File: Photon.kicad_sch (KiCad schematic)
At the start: 58 parts, among them J1 USB_C_Receptacle_USB2.0_14P, Q1 IRLML6402, Q2 IRLML6402, SW1 TS-1088-AR02016, U1 ATtiny13A-S, U2 RT8059GJ5, U3 TP4056, U4 BCR421UW6-7, U5 DW01A, U6 FS8205A, U7 BCR421UW6-7

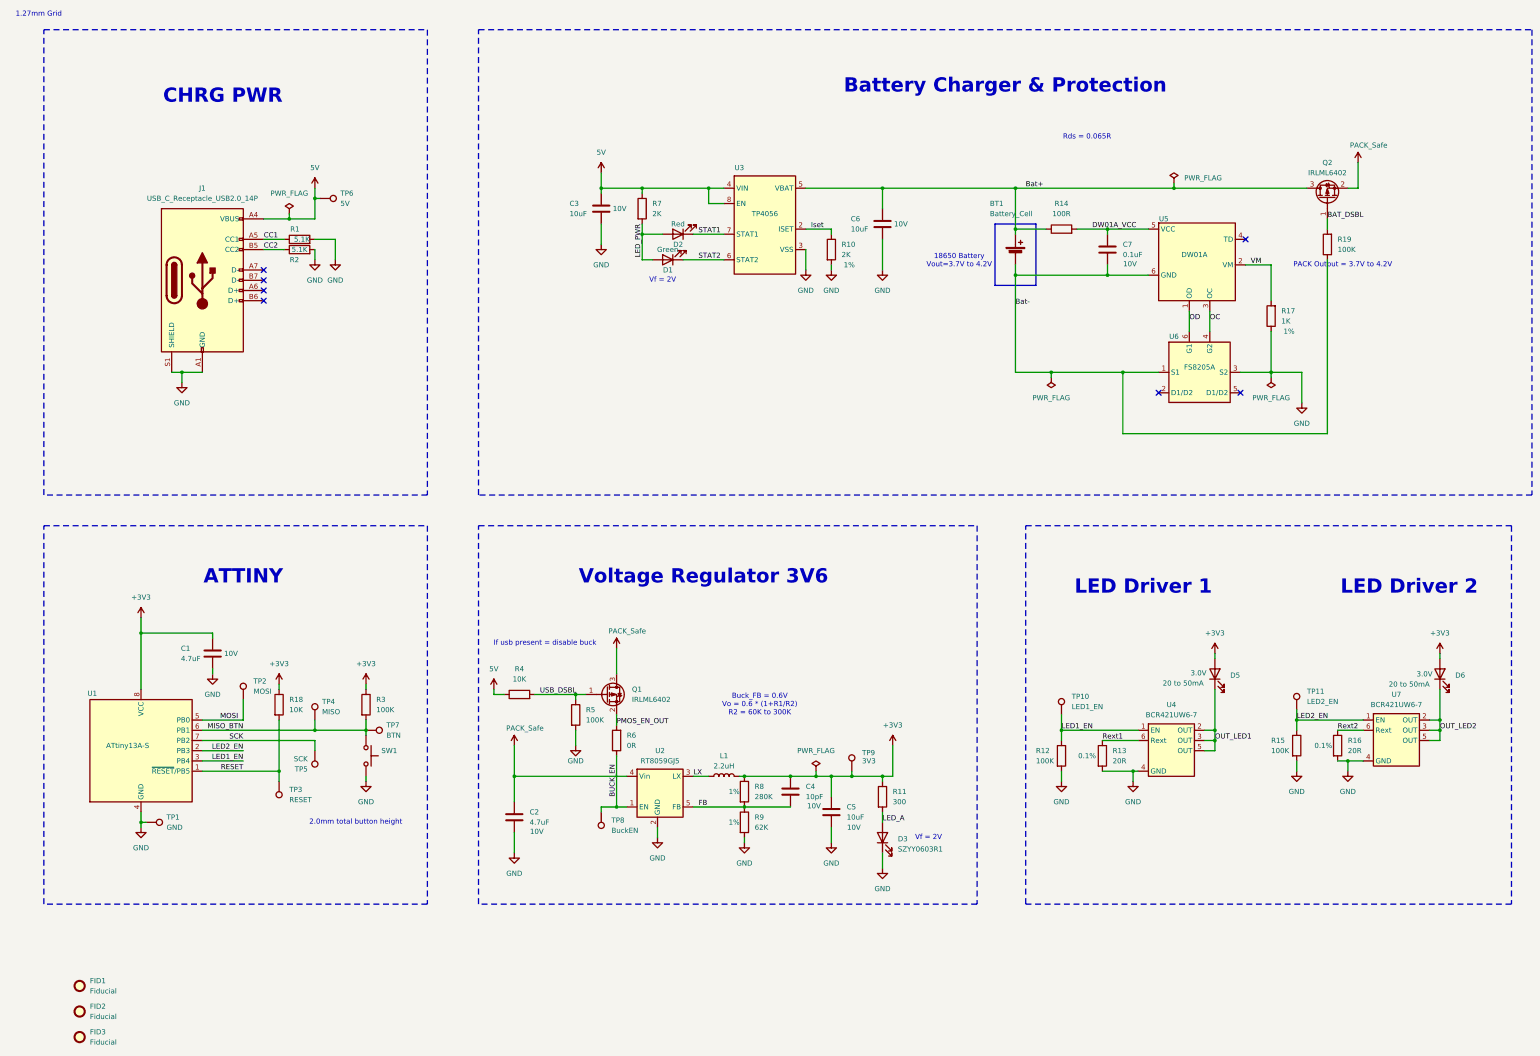
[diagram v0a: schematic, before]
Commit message: Cleaned up PCB
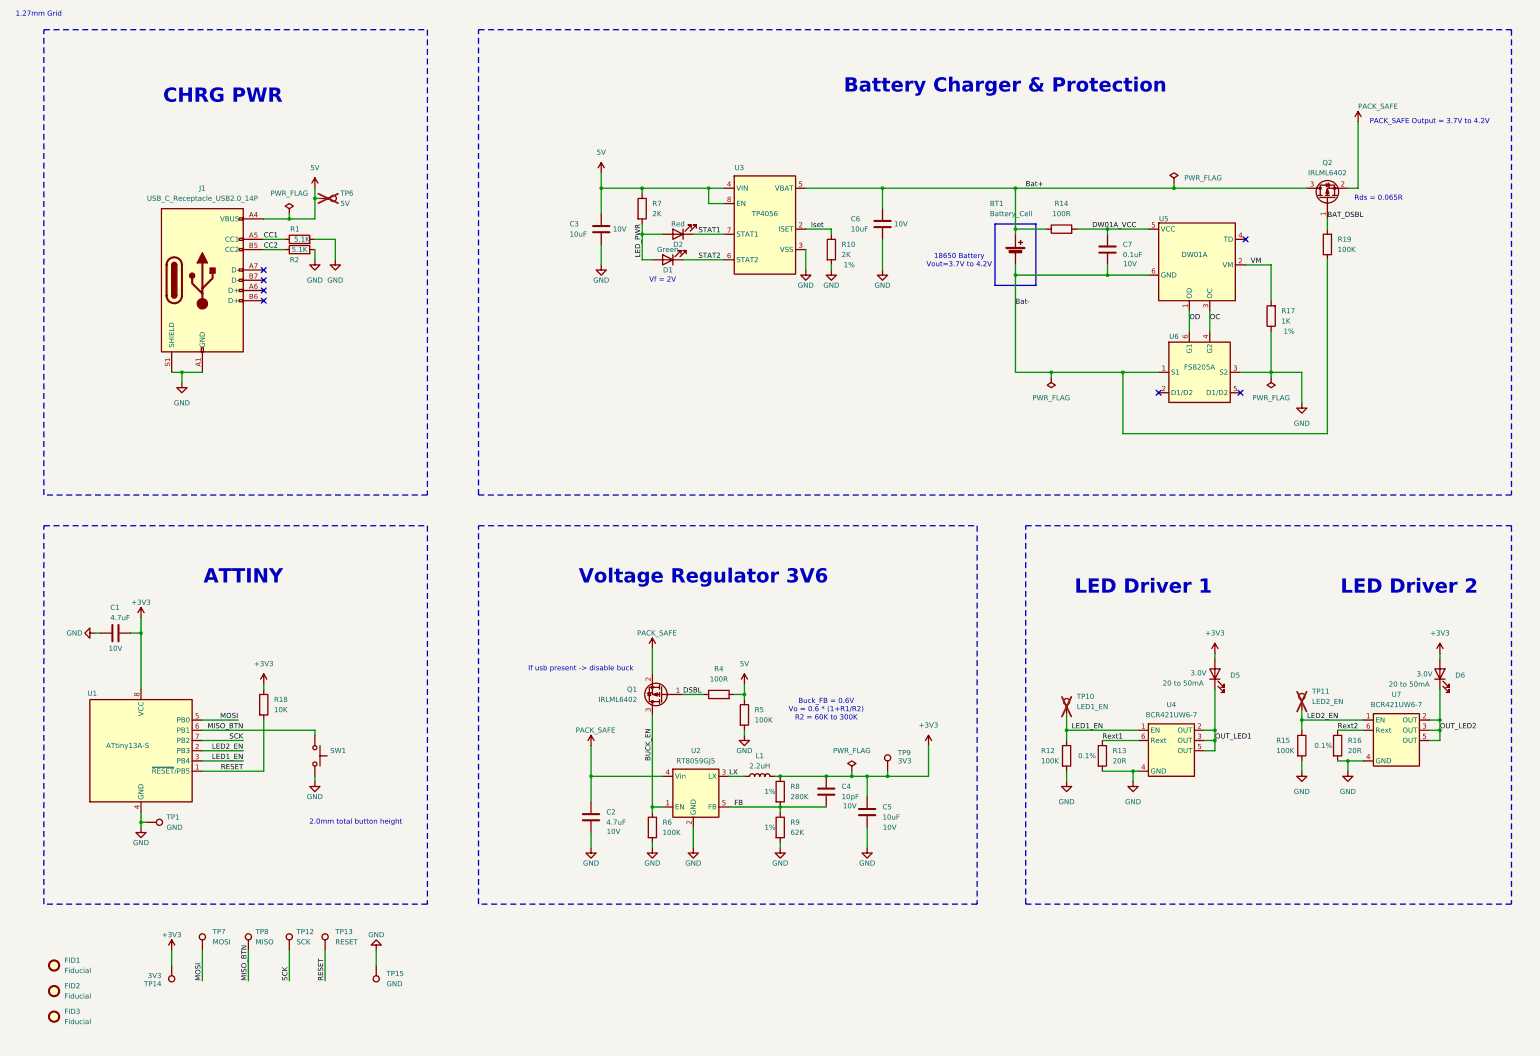
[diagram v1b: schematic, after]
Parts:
- removed D3: SZYY0603R1, LED_SMD:LED_0603_1608Metric, symbol Device:LED
- removed R11: 300, Resistor_SMD:R_0603_1608Metric, symbol Device:R
- removed R3: 100K, Resistor_SMD:R_0603_1608Metric, symbol Device:R
- removed TP2: MOSI, TestPoint:TestPoint_Pad_D1.0mm, symbol Connector:TestPoint
- removed TP3: RESET, TestPoint:TestPoint_Pad_D1.0mm, symbol Connector:TestPoint
- removed TP4: MISO, TestPoint:TestPoint_Pad_D1.0mm, symbol Connector:TestPoint
- removed TP5: SCK, TestPoint:TestPoint_Pad_D1.0mm, symbol Connector:TestPoint
- added TP12: SCK, TestPoint:TestPoint_Pad_D1.0mm, symbol Connector:TestPoint
- added TP13: RESET, TestPoint:TestPoint_Pad_D1.0mm, symbol Connector:TestPoint
- added TP14: 3V3, TestPoint:TestPoint_THTPad_D1.0mm_Drill0.5mm, symbol Connector:TestPoint
- added TP15: GND, TestPoint:TestPoint_Pad_D1.0mm, symbol Connector:TestPoint
- BT1: footprint Photon:18650 Battery Holder -> Photon:Spring Battery TH
- R4: value 10K -> 100R
- R6: value 0R -> 100K
- TP10, TP11, TP6: footprint TestPoint:TestPoint_Pad_D1.0mm -> TestPoint:TestPoint_THTPad_D1.0mm_Drill0.5mm; now not fitted
- TP7: value BTN -> MOSI
- TP8: value BuckEN -> MISO
- U4, U5, U6, U7: footprint Package_TO_SOT_SMD:SOT-23-6_Handsoldering -> Package_TO_SOT_SMD:SOT-23-6
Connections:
- net +3V3: now also TP14.1
- net 5V: now also R4.2, R5.1; no longer R4.1
- net BUCK_EN: now also Q1.3 (D); no longer TP8.1
- net GND: now also R6.2, TP15.1
- net MISO_BTN: now also TP8.1; no longer TP7.1
- net MOSI: now also TP7.1
- net RESET: now also TP13.1
- net SCK: now also TP12.1
- net PACK_Safe renamed PACK_SAFE
- net PACK_SAFE: now also Q1.2 (S); no longer Q1.3 (D)
- removed net PMOS_EN_OUT: Q1.2 (S), R6.2
- removed net USB_DSBL: Q1.1 (G), R4.2, R5.1
- new net DSBL: Q1.1 (G), R4.1
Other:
- note added: "If usb present -> disable buck"
- note added: "PACK_SAFE Output = 3.7V to 4.2V"
- note removed: "If usb present = disable buck"
- note removed: "PACK Output = 3.7V to 4.2V"
- moved on the sheet: C1, C2, C3, C4, C5, FID1, FID2, FID3, L1, Q1, R12, R15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
